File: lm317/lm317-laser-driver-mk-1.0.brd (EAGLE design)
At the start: 24.1 x 21.6 mm, 8 parts, among them U1 LM317

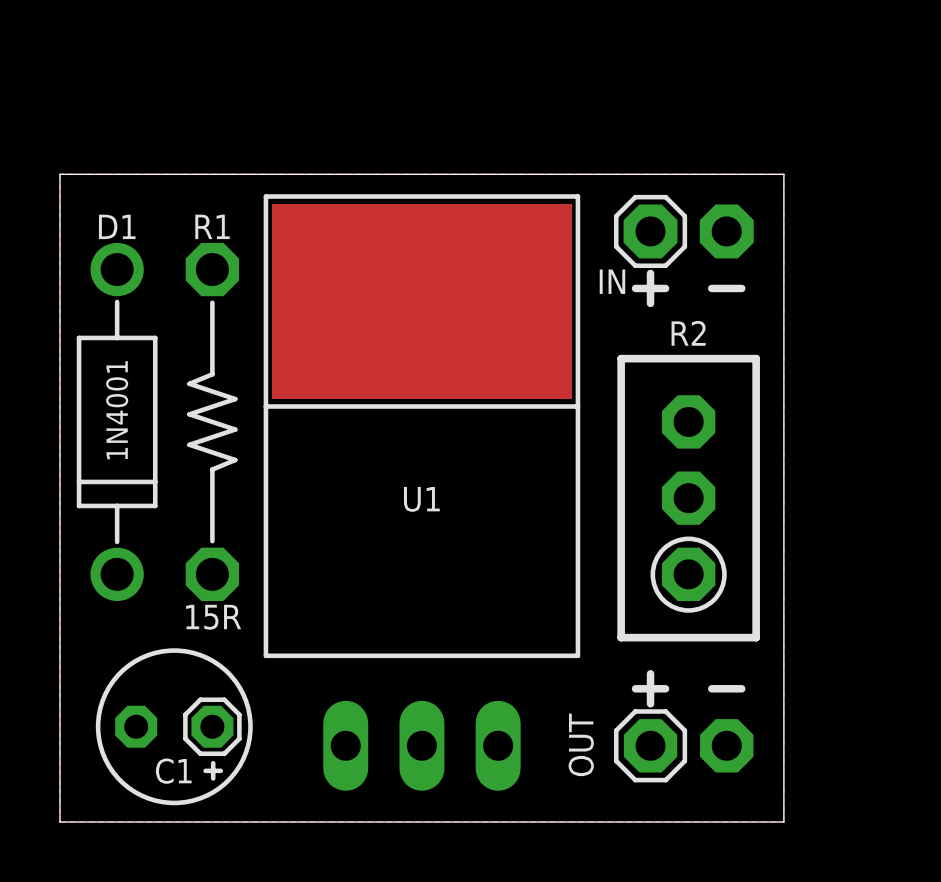
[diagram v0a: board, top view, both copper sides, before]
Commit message: wip
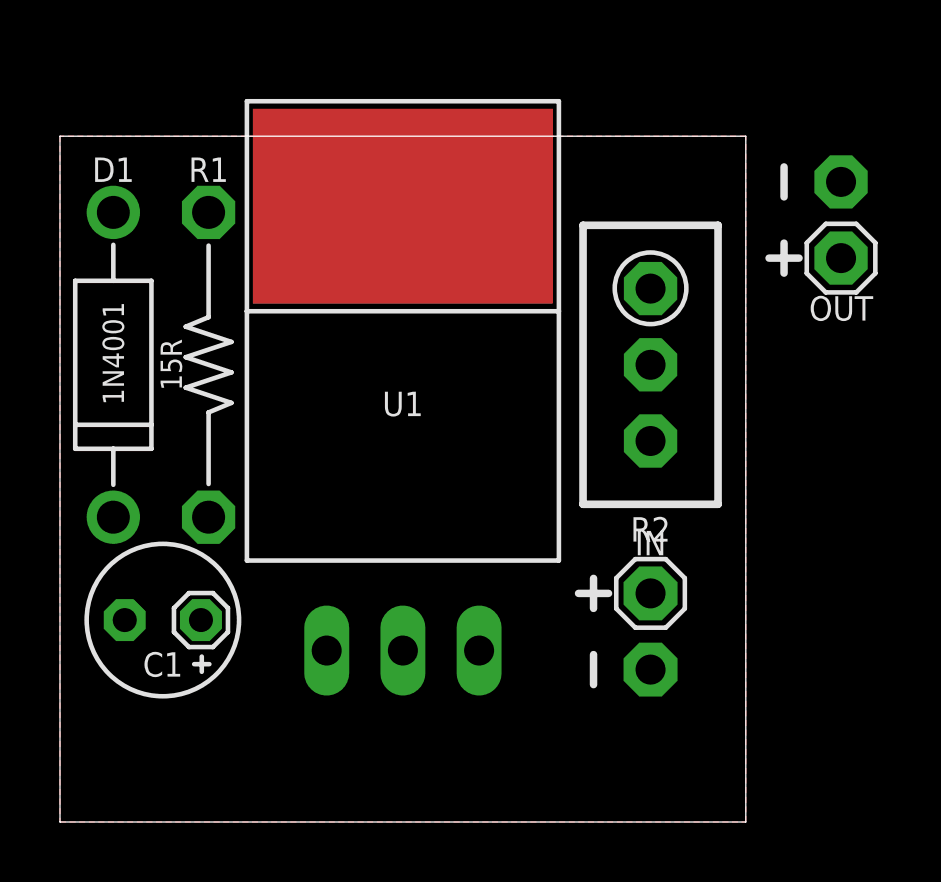
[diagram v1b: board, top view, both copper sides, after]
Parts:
- moved OUT 18.2 mm to (26.0, 20.1), turned to 270 degrees
- moved IN 13.4 mm to (19.7, 6.35), turned to 270 degrees
- moved R2 4.62 mm to (19.7, 15.2), turned to 270 degrees
- moved C1 3.58 mm to (3.43, 6.73)
- moved U1 3.24 mm to (11.4, 5.71)
- moved D1 1.91 mm to (1.78, 15.2)
- moved R1 1.91 mm to (4.95, 15.2)
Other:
- board size 24.1 x 21.6 mm -> 22.9 x 22.9 mm
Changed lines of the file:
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@@
 <setting verticaltext="up"/>
 </settings>
-<grid distance="25" unitdist="mil" unit="mil" style="lines" multiple="4" display="yes" altdistance="1" altunitdist="mil" altunit="mil"/>
+<grid distance="5" unitdist="mil" unit="mil" style="lines" multiple="5" display="yes" altdistance="1" altunitdist="mil" altunit="mil"/>
 <layers>
 <layer number="1" name="Top" color="4" fill="1" visible="yes" active="yes"/>
@@
 <board>
 <plain>
-<wire x1="0" y1="0" x2="24.13" y2="0" width="0" layer="20"/>
-<wire x1="24.13" y1="0" x2="24.13" y2="21.59" width="0" layer="20"/>
-<wire x1="24.13" y1="21.59" x2="0" y2="21.59" width="0" layer="20"/>
-<wire x1="0" y1="21.59" x2="0" y2="0" width="0" layer="20"/>
+<wire x1="0" y1="0" x2="22.86" y2="0" width="0" layer="20"/>
+<wire x1="22.86" y1="0" x2="22.86" y2="22.86" width="0" layer="20"/>
+<wire x1="22.86" y1="22.86" x2="0" y2="22.86" width="0" layer="20"/>
+<wire x1="0" y1="22.86" x2="0" y2="0" width="0" layer="20"/>
 </plain>
 <attributes>
@@
 <attribute name="DESIGNER" value="sean@yak.net" x="13.97" y="-1.27" size="1.778" layer="27" display="off"/>
 </element>
-<element name="C1" library="a_parts" package="E2,5-5" value="10uF" x="3.81" y="3.175" smashed="yes" rot="R180">
-<attribute name="NAME" x="3.81" y="2.102" size="0.8128" layer="25" font="vector" ratio="10" rot="R180" align="bottom-center"/>
-<attribute name="VALUE" x="3.81" y="4.248" size="0.7112" layer="27" font="vector" ratio="10" rot="R180" align="top-center"/>
-</element>
-<element name="R1" library="a_parts" package="RESISTOR-AXIAL-PTH-10.16MM" value="15R" x="5.08" y="13.335" smashed="yes" rot="R270">
-<attribute name="NAME" x="5.08" y="19.431" size="0.8128" layer="25" font="vector" ratio="10" align="bottom-center"/>
-<attribute name="VALUE" x="5.08" y="7.239" size="0.8128" layer="21" font="vector" ratio="10" rot="R180" align="bottom-center"/>
-</element>
-<element name="R2" library="a_parts" package="RTRIM3296W" value="1K" x="20.955" y="10.795" smashed="yes" rot="R90">
-<attribute name="NAME" x="20.955" y="15.875" size="0.8128" layer="25" font="vector" ratio="12" align="bottom-center"/>
-<attribute name="VALUE" x="20.955" y="5.715" size="0.8128" layer="27" font="vector" ratio="12" rot="R180" align="bottom-center"/>
-</element>
-<element name="D1" library="a_parts" package="DIODE-10.16MM-NOSYMBOL" value="1N4001" x="1.905" y="13.335" smashed="yes" rot="R270">
-<attribute name="NAME" x="1.905" y="19.431" size="0.8128" layer="25" font="vector" ratio="10" align="bottom-center"/>
-<attribute name="VALUE" x="1.905" y="13.716" size="0.7112" layer="21" font="vector" ratio="10" rot="R270" align="center"/>
-</element>
-<element name="U1" library="a_parts" package="TO220-THERMPAD" value="LM317" x="12.065" y="2.54" smashed="yes">
-<attribute name="NAME" x="12.065" y="10.355" size="0.8128" layer="25" font="vector" ratio="10" align="bottom-center"/>
-<attribute name="VALUE" x="12.165" y="9.55" size="0.8128" layer="27" font="vector" ratio="10" align="center"/>
-</element>
-<element name="IN" library="a_parts" package="1X02-CENTER-L+" value="M02PTH-CENTERED-L+" x="20.955" y="19.685" smashed="yes">
-<attribute name="NAME" x="18.415" y="18.415" size="0.8128" layer="25" font="vector" ratio="10" rot="R180" align="bottom-center"/>
-</element>
-<element name="OUT" library="a_parts" package="1X02-CENTER-R+" value="M02PTH-CENTERED-R+" x="20.955" y="2.54" smashed="yes" rot="R180">
-<attribute name="NAME" x="17.78" y="2.54" size="0.8128" layer="25" font="vector" ratio="10" rot="R90" align="bottom-center"/>
+<element name="C1" library="a_parts" package="E2,5-5" value="10uF" x="3.429" y="6.731" smashed="yes" rot="R180">
+<attribute name="NAME" x="3.429" y="5.658" size="0.8128" layer="25" font="vector" ratio="10" rot="R180" align="bottom-center"/>
+<attribute name="VALUE" x="3.429" y="7.931" size="0.7112" layer="27" font="vector" ratio="10" rot="R180" align="top-center"/>
+</element>
+<element name="R1" library="a_parts" package="RESISTOR-AXIAL-PTH-10.16MM" value="15R" x="4.953" y="15.24" smashed="yes" rot="R270">
+<attribute name="NAME" x="4.953" y="21.336" size="0.8128" layer="25" font="vector" ratio="10" align="bottom-center"/>
+<attribute name="VALUE" x="4.064" y="15.24" size="0.7112" layer="21" font="vector" ratio="10" rot="R90" align="bottom-center"/>
+</element>
+<element name="R2" library="a_parts" package="RTRIM3296W" value="1K" x="19.685" y="15.24" smashed="yes" rot="R270">
+<attribute name="NAME" x="19.685" y="10.16" size="0.8128" layer="25" font="vector" ratio="12" rot="R180" align="bottom-center"/>
+<attribute name="VALUE" x="19.685" y="20.32" size="0.8128" layer="27" font="vector" ratio="12" align="bottom-center"/>
+</element>
+<element name="D1" library="a_parts" package="DIODE-10.16MM-NOSYMBOL" value="1N4001" x="1.778" y="15.24" smashed="yes" rot="R270">
+<attribute name="NAME" x="1.778" y="21.336" size="0.8128" layer="25" font="vector" ratio="10" align="bottom-center"/>
+<attribute name="VALUE" x="1.778" y="15.621" size="0.7112" layer="21" font="vector" ratio="10" rot="R270" align="center"/>
+</element>
+<element name="U1" library="a_parts" package="TO220-THERMPAD" value="LM317" x="11.43" y="5.715" smashed="yes">
+<attribute name="NAME" x="11.43" y="13.53" size="0.8128" layer="25" font="vector" ratio="10" align="bottom-center"/>
+<attribute name="VALUE" x="11.53" y="12.725" size="0.8128" layer="27" font="vector" ratio="10" align="center"/>
+</element>
+<element name="IN" library="a_parts" package="1X02-CENTER-L+" value="M02PTH-CENTERED-L+" x="19.685" y="6.35" smashed="yes" rot="R270">
+<attribute name="NAME" x="19.685" y="8.89" size="0.8128" layer="25" font="vector" ratio="10" align="bottom-center"/>
+</element>
+<element name="OUT" library="a_parts" package="1X02-CENTER-R+" value="M02PTH-CENTERED-R+" x="26.035" y="20.066" smashed="yes" rot="R270">
+<attribute name="NAME" x="26.035" y="17.526" size="0.8128" layer="25" font="vector" ratio="10" rot="R180" align="bottom-center"/>
 </element>
 </elements>
@@
 <polygon width="0.1524" layer="1">
 <vertex x="0" y="0"/>
-<vertex x="24.13" y="0"/>
-<vertex x="24.13" y="21.59"/>
-<vertex x="0" y="21.59"/>
+<vertex x="22.86" y="0"/>
+<vertex x="22.86" y="22.86"/>
+<vertex x="0" y="22.86"/>
 </polygon>
 </signal>
@@
 <contactref element="IN" pad="1"/>
 <contactref element="U1" pad="3"/>
-<wire x1="14.605" y1="2.54" x2="19.685" y2="19.685" width="0" layer="19" extent="1-1"/>
+<wire x1="19.685" y1="7.62" x2="13.97" y2="5.715" width="0" layer="19" extent="1-1"/>
 </signal>
 <signal name="N$2">
@@
 <contactref element="U1" pad="2@2" route="any" routetag="G$1.OUT"/>
 <contactref element="R1" pad="P$1"/>
-<wire x1="12.065" y1="17.35" x2="5.08" y2="18.415" width="0" layer="19" extent="1-1"/>
+<wire x1="11.43" y1="20.525" x2="4.953" y2="20.32" width="0" layer="19" extent="1-1"/>
 </signal>
 <signal name="N$3">
 <contactref element="R1" pad="P$2"/>
 <contactref element="R2" pad="1"/>
-<wire x1="5.08" y1="8.255" x2="20.955" y2="8.255" width="0" layer="19" extent="1-1"/>
+<wire x1="4.953" y1="10.16" x2="19.685" y2="17.78" width="0" layer="19" extent="1-1"/>
 </signal>
 <signal name="OUT">
@@
 <contactref element="C1" pad="+"/>
 <contactref element="R2" pad="2"/>
-<wire x1="19.685" y1="2.54" x2="20.955" y2="10.795" width="0" layer="19" extent="1-1"/>
-<wire x1="9.525" y1="2.54" x2="19.685" y2="2.54" width="0" layer="19" extent="1-1"/>
-<wire x1="5.08" y1="3.175" x2="9.525" y2="2.54" width="0" layer="19" extent="1-1"/>
-<wire x1="1.905" y1="8.255" x2="5.08" y2="3.175" width="0" layer="19" extent="1-1"/>
+<wire x1="8.89" y1="5.715" x2="19.685" y2="15.24" width="0" layer="19" extent="1-1"/>
+<wire x1="4.699" y1="6.731" x2="8.89" y2="5.715" width="0" layer="19" extent="1-1"/>
+<wire x1="1.778" y1="10.16" x2="4.699" y2="6.731" width="0" layer="19" extent="1-1"/>
+<wire x1="26.035" y1="18.796" x2="4.699" y2="6.731" width="0" layer="19" extent="1-1"/>
 </signal>
 </signals>

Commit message: uncommitted pcb revs
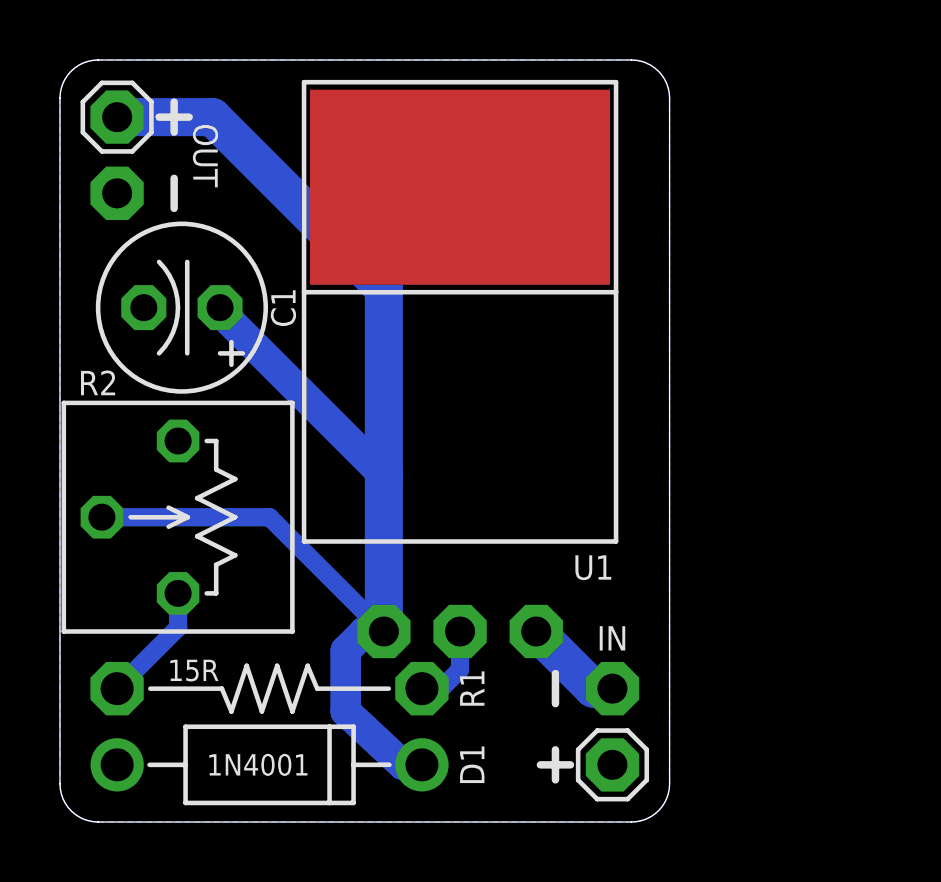
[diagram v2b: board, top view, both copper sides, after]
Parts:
- added U$1: (no value), a_parts:COW
- C1: device a_parts:E2,5-5 -> a_parts:E2,5-6
- IN: value M02PTH-CENTERED-L+ -> M02PTH-CENTERED-R+; device a_parts:1X02-CENTER-L+ -> a_parts:1X02-CENTER-R+
- R2: value 1K -> 0-1K; device a_parts:RTRIM3296W -> a_parts:TRIM_POT_PTH2
- moved OUT 24.2 mm to (1.91, 22.2), turned to 90 degrees
- moved R2 16.5 mm to (3.94, 10.2), turned to 90 degrees
- moved D1 14.3 mm to (6.99, 1.91), turned to 0 degrees
- moved R1 11.0 mm to (6.99, 4.45), turned to 180 degrees
- moved C1 10.4 mm to (4.06, 17.1)
- moved IN 3.42 mm to (18.4, 3.17)
- moved U1 2.01 mm to (13.3, 6.35)
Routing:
- net OUT: track 0.00 -> 48.3 mm
- net N$1: track 0.00 -> 4.02 mm
- net VCC: track 0.00 -> 3.33 mm
- net N$2: track 0.00 -> 2.80 mm
- added copper zone on layer 16, net GND
- removed copper zone on layer 1, net GND
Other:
- board size 22.9 x 22.9 mm -> 20.3 x 25.4 mm
- board text added: ">VERSION"
- board text added: "LM317 Laser Driver"
